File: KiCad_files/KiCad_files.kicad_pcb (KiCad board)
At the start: 2 copper layers, 82 x 102 mm, 76 parts, among them J1 Conn_01x02_Socket, J2 L717HDE15P, J3 Conn_01x03_Socket, SW1 WE430182070816, U1 LM22670QMR-5.0, U2 MC33275ST-3.3T3G, U3 ADM3488ExR, U6 LT1789

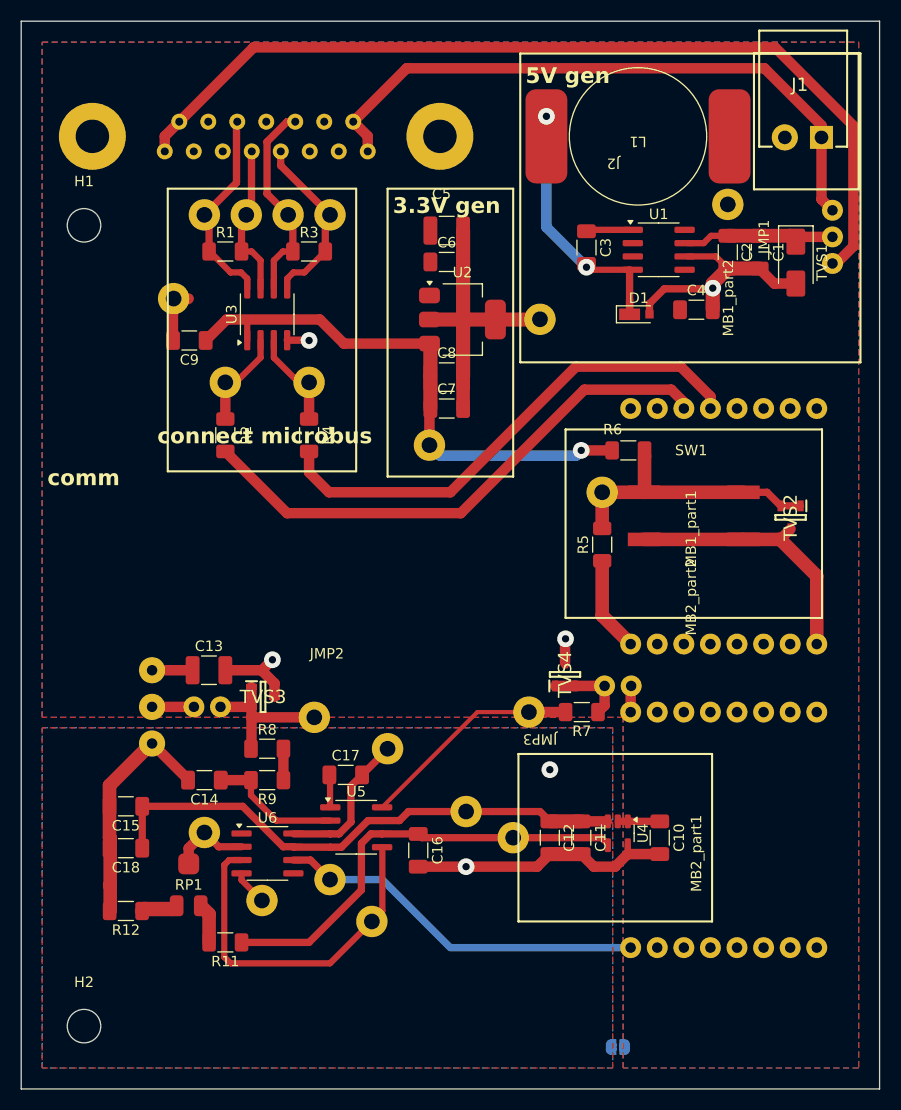
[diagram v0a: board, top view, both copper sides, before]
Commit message: Unremarkable changes
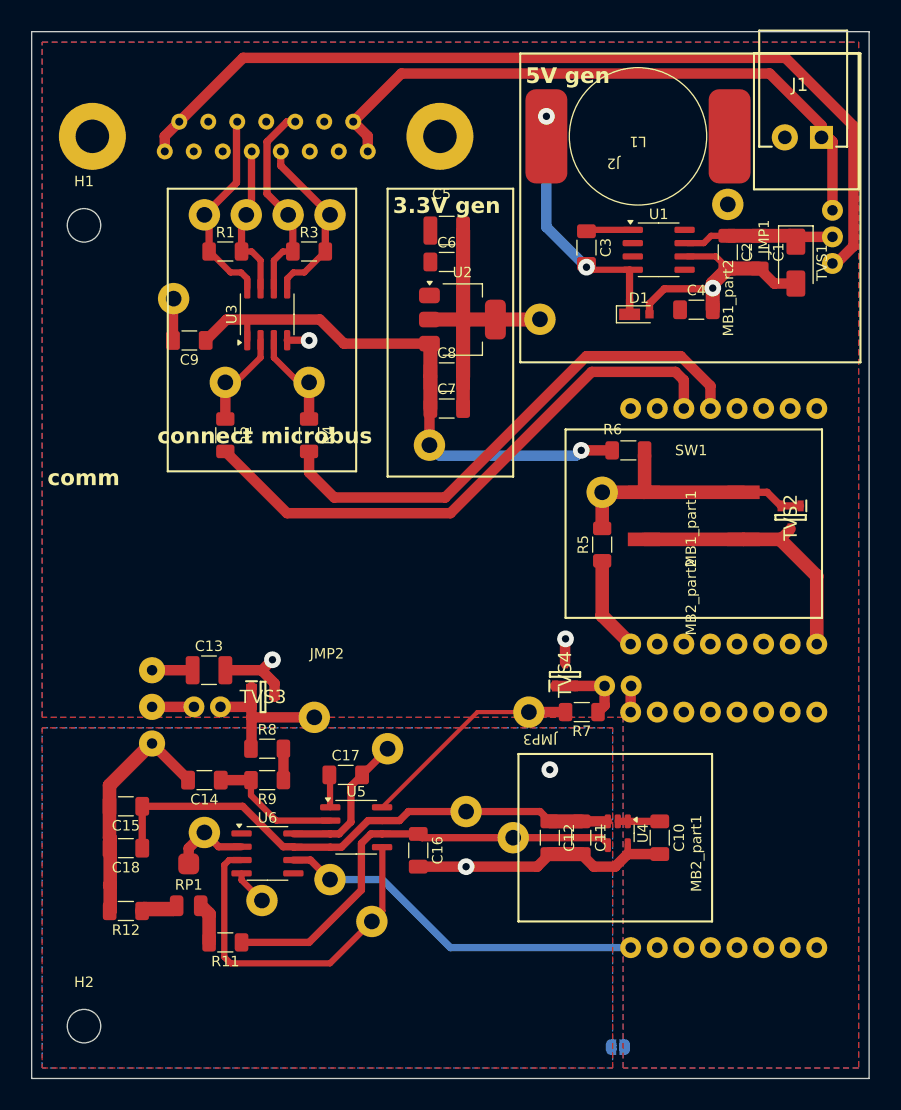
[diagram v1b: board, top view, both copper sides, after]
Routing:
- net /MB1_14: track 52.2 -> 54.9 mm
- net /MB1_13: track 48.4 -> 50.3 mm
- net /15: track 88.0 -> 87.2 mm
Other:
- board size 82 x 102 mm -> 80 x 100 mm
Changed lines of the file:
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@@
 	)
 	(gr_line
-		(start 201 141)
-		(end 201 39)
+		(start 200 140)
+		(end 200 40)
 		(stroke
 			(width 0.05)
@@
 	)
 	(gr_line
-		(start 119 39)
-		(end 119 141)
+		(start 120 40)
+		(end 120 140)
 		(stroke
 			(width 0.05)
@@
 	)
 	(gr_line
-		(start 201 141)
-		(end 119 141)
+		(start 200 140)
+		(end 120 140)
 		(stroke
 			(width 0.05)
@@
 	)
 	(gr_line
-		(start 119 39)
-		(end 201 39)
+		(start 120 40)
+		(end 200 40)
 		(stroke
 			(width 0.05)
@@
 	)
 	(segment
+		(start 198.5 60.5)
+		(end 198.5 49)
+		(width 1)
+		(layer "F.Cu")
+		(net 9)
+	)
+	(segment
+		(start 192 42.5)
+		(end 140.2 42.5)
+		(width 1)
+		(layer "F.Cu")
+		(net 9)
+	)
+	(segment
+		(start 132.715 49.985)
+		(end 132.715 51.44)
+		(width 1)
+		(layer "F.Cu")
+		(net 9)
+	)
+	(segment
+		(start 140.2 42.5)
+		(end 134.1 48.6)
+		(width 1)
+		(layer "F.Cu")
+		(net 9)
+	)
+	(segment
+		(start 196.8575 62.1425)
+		(end 198.5 60.5)
+		(width 1)
+		(layer "F.Cu")
+		(net 9)
+	)
+	(segment
+		(start 198.5 49)
+		(end 192 42.5)
+		(width 1)
+		(layer "F.Cu")
+		(net 9)
+	)
+	(segment
+		(start 134.1 48.6)
+		(end 132.715 49.985)
+		(width 1)
+		(layer "F.Cu")
+		(net 9)
+	)
+	(segment
 		(start 196.5 62.1425)
 		(end 196.8575 62.1425)
@@
 	)
 	(segment
-		(start 132.715 49.985)
-		(end 132.715 51.44)
-		(width 1)
-		(layer "F.Cu")
-		(net 9)
-	)
-	(segment
-		(start 196.8575 62.1425)
-		(end 198.5 60.5)
-		(width 1)
-		(layer "F.Cu")
-		(net 9)
-	)
-	(segment
-		(start 141.2 41.5)
-		(end 134.1 48.6)
-		(width 1)
-		(layer "F.Cu")
-		(net 9)
-	)
-	(segment
-		(start 198.5 49)
-		(end 191 41.5)
-		(width 1)
-		(layer "F.Cu")
-		(net 9)
-	)
-	(segment
-		(start 134.1 48.6)
-		(end 132.715 49.985)
-		(width 1)
-		(layer "F.Cu")
-		(net 9)
-	)
-	(segment
-		(start 198.5 60.5)
-		(end 198.5 49)
-		(width 1)
-		(layer "F.Cu")
-		(net 9)
-	)
-	(segment
-		(start 191 41.5)
-		(end 141.2 41.5)
-		(width 1)
-		(layer "F.Cu")
-		(net 9)
-	)
-	(segment
 		(start 146.05 63)
 		(end 148.05 61)
@@
 	)
 	(segment
+		(start 144.5 57.5)
+		(end 142.483 55.483)
+		(width 0.7)
+		(layer "F.Cu")
+		(net 12)
+	)
+	(segment
+		(start 142.483 50.517)
+		(end 144.4 48.6)
+		(width 0.7)
+		(layer "F.Cu")
+		(net 12)
+	)
+	(segment
+		(start 144.95 61)
+		(end 144.95 57.95)
+		(width 0.7)
+		(layer "F.Cu")
+		(net 12)
+	)
+	(segment
+		(start 144 61)
+		(end 144.95 61)
+		(width 0.6)
+		(layer "F.Cu")
+		(net 12)
+	)
+	(segment
+		(start 144.4 48.6)
+		(end 145.18 48.6)
+		(width 0.7)
+		(layer "F.Cu")
+		(net 12)
+	)
+	(segment
+		(start 144.95 57.95)
+		(end 144.5 57.5)
+		(width 0.7)
+		(layer "F.Cu")
+		(net 12)
+	)
+	(segment
 		(start 142.483 55.483)
 		(end 142.483 50.517)
@@
 	)
 	(segment
-		(start 144.95 61)
-		(end 144.95 57.95)
-		(width 0.7)
-		(layer "F.Cu")
-		(net 12)
-	)
-	(segment
-		(start 144 61)
-		(end 144.95 61)
-		(width 0.6)
-		(layer "F.Cu")
-		(net 12)
-	)
-	(segment
-		(start 142.483 50.517)
-		(end 144.4 48.6)
-		(width 0.7)
-		(layer "F.Cu")
-		(net 12)
-	)
-	(segment
-		(start 144.95 57.95)
-		(end 144.5 57.5)
-		(width 0.7)
-		(layer "F.Cu")
-		(net 12)
-	)
-	(segment
 		(start 143.135 64.525)
 		(end 143.135 61.865)
@@
 	)
 	(segment
-		(start 144.5 57.5)
-		(end 142.483 55.483)
-		(width 0.7)
-		(layer "F.Cu")
-		(net 12)
-	)
-	(segment
-		(start 144.4 48.6)
-		(end 145.18 48.6)
-		(width 0.7)
-		(layer "F.Cu")
-		(net 12)
-	)
-	(segment
 		(start 143.135 61.865)
 		(end 144 61)
@@
 	)
 	(segment
+		(start 190.5 44)
+		(end 155.32 44)
+		(width 1)
+		(layer "F.Cu")
+		(net 13)
+	)
+	(segment
 		(start 150.72 48.6)
 		(end 152.105 49.985)
@@
 	)
 	(segment
-		(start 195.45 48.95)
-		(end 190 43.5)
-		(width 1)
-		(layer "F.Cu")
-		(net 13)
-	)
-	(segment
 		(start 195.45 50.1)
 		(end 195.45 48.95)
@@
 	)
 	(segment
-		(start 195.45 56.0125)
+		(start 155.32 44)
+		(end 150.72 48.6)
+		(width 1)
+		(layer "F.Cu")
+		(net 13)
+	)
+	(segment
+		(start 195.45 50.1)
+		(end 196.1 50.1)
+		(width 1)
+		(layer "F.Cu")
+		(net 13)
+	)
+	(segment
+		(start 195.45 48.95)
+		(end 190.5 44)
+		(width 1)
+		(layer "F.Cu")
+		(net 13)
+	)
+	(segment
+		(start 196.5 50.5)
 		(end 196.5 57.0625)
 		(width 1)
@@
 	)
 	(segment
-		(start 155.82 43.5)
-		(end 150.72 48.6)
-		(width 1)
-		(layer "F.Cu")
-		(net 13)
-	)
-	(segment
-		(start 195.45 50.1)
-		(end 195.45 56.0125)
-		(width 1)
-		(layer "F.Cu")
-		(net 13)
-	)
-	(segment
-		(start 190 43.5)
-		(end 155.82 43.5)
+		(start 196.1 50.1)
+		(end 196.5 50.5)
 		(width 1)
 		(layer "F.Cu")
@@
 	)
 	(segment
-		(start 161 86)
-		(end 172.8 74.2)
+		(start 160 86)
+		(end 173.5 72.5)
 		(width 1)
 		(layer "F.Cu")
@@
 	)
 	(segment
-		(start 182.3 75.4)
+		(start 181.5 72.5)
+		(end 182.3 73.3)
+		(width 1)
+		(layer "F.Cu")
+		(net 26)
+	)
+	(segment
+		(start 182.3 73.3)
 		(end 182.3 76)
 		(width 1)
@@
 	)
 	(segment
-		(start 144.4 86)
-		(end 161 86)
+		(start 173.5 72.5)
+		(end 181.5 72.5)
 		(width 1)
 		(layer "F.Cu")
@@
 	)
 	(segment
-		(start 181.1 74.2)
-		(end 182.3 75.4)
+		(start 144.4 86)
+		(end 160 86)
 		(width 1)
 		(layer "F.Cu")
@@
 	)
 	(segment
-		(start 172.8 74.2)
-		(end 181.1 74.2)
-		(width 1)
-		(layer "F.Cu")
-		(net 26)
-	)
-	(segment
-		(start 172 72)
-		(end 182 72)
+		(start 148.9 84.5)
+		(end 159.5 84.5)
 		(width 1)
 		(layer "F.Cu")
@@
 	)
 	(segment
-		(start 182 72)
-		(end 184.84 74.84)
+		(start 182 71)
+		(end 184.84 73.84)
 		(width 1)
 		(layer "F.Cu")
@@
 	)
 	(segment
+		(start 184.84 73.84)
+		(end 184.84 76)
+		(width 1)
+		(layer "F.Cu")
+		(net 27)
+	)
+	(segment
+		(start 159.5 84.5)
+		(end 173 71)
+		(width 1)
+		(layer "F.Cu")
+		(net 27)
+	)
+	(segment
+		(start 173 71)
+		(end 182 71)
+		(width 1)
+		(layer "F.Cu")
+		(net 27)
+	)
+	(segment
 		(start 146.5 82.1)
-		(end 148.4 84)
-		(width 1)
-		(layer "F.Cu")
-		(net 27)
-	)
-	(segment
-		(start 184.84 74.84)
-		(end 184.84 76)
+		(end 148.9 84.5)
 		(width 1)
 		(layer "F.Cu")
@@
 		(start 146.5 80.1)
 		(end 146.5 82.1)
-		(width 1)
-		(layer "F.Cu")
-		(net 27)
-	)
-	(segment
-		(start 160 84)
-		(end 172 72)
-		(width 1)
-		(layer "F.Cu")
-		(net 27)
-	)
-	(segment
-		(start 148.4 84)
-		(end 160 84)
 		(width 1)
 		(layer "F.Cu")
@@
 		(layer "F.Cu")
 		(net 55)
-	)
-	(segment
-		(start 134.9375 65.5625)
-		(end 135 65.5)
-		(width 1)
-		(layer "F.Cu")
-		(net 55)
